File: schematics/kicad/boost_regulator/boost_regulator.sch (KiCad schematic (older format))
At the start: 5 parts, among them SW1 

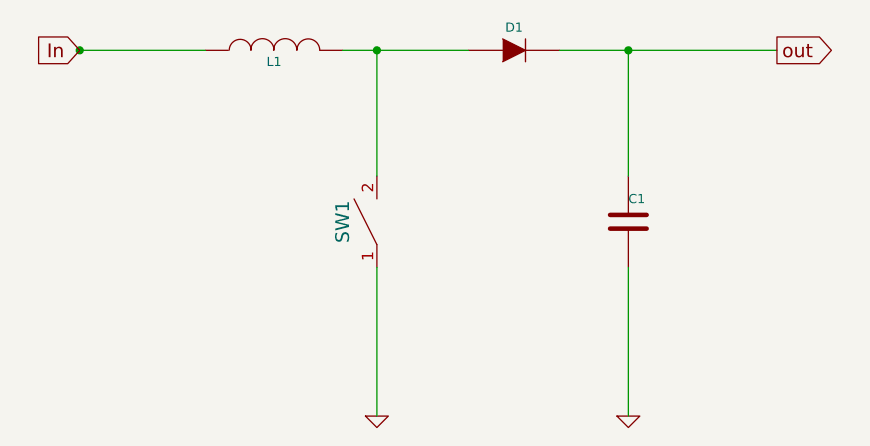
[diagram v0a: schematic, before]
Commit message: schéma jolis pour les screenshot, et screenshots
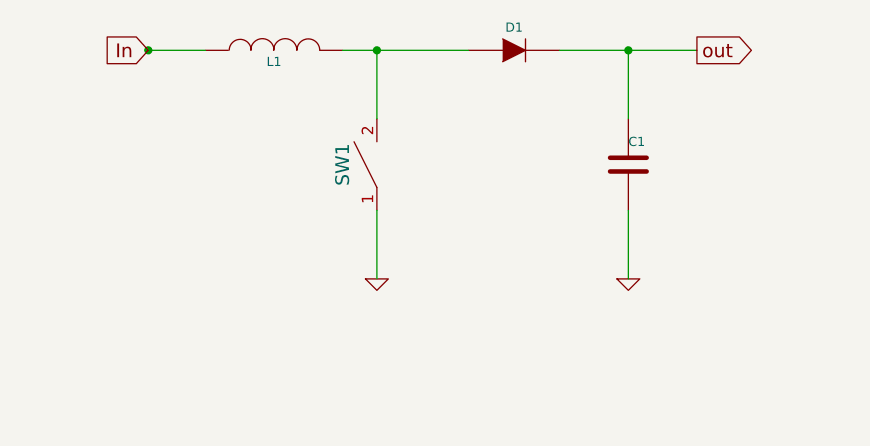
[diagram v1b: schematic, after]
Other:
- moved on the sheet: C1, SW1
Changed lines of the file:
@@
 Sheet 1 1
 Title ""
-Date "8 sep 2015"
+Date "12 sep 2015"
 Rev ""
 Comp ""
@@
 Comment4 ""
 $EndDescr
-Connection ~ 2100 2450
-Text GLabel 2100 2450 0    60   Input ~ 0
+Connection ~ 2400 2450
+Text GLabel 2400 2450 0    60   Input ~ 0
 In
 $Comp
@@
 L C C1
 U 1 1 55EDF250
-P 4500 3200
-F 0 "C1" H 4500 3300 40  0000 L CNN
-F 1 " " H 4506 3115 40  0000 L CNN
-F 2 "~" H 4538 3050 30  0000 C CNN
-F 3 "~" H 4500 3200 60  0000 C CNN
-	1    4500 3200
+P 4500 2950
+F 0 "C1" H 4500 3050 40  0000 L CNN
+F 1 " " H 4506 2865 40  0000 L CNN
+F 2 "~" H 4538 2800 30  0000 C CNN
+F 3 "~" H 4500 2950 60  0000 C CNN
+	1    4500 2950
 	1    0    0    -1
 $EndComp
-Text GLabel 5150 2450 2    60   Output ~ 0
+Text GLabel 4800 2450 2    60   Output ~ 0
 out
 $Comp
 L GND GND
 U 1 1 55EDF277
-P 3400 4050
-F 0 "GND" H 3400 4050 30  0001 C CNN
-F 1 "GND" H 3400 3980 30  0001 C CNN
-F 2 "" H 3400 4050 60  0000 C CNN
-F 3 "" H 3400 4050 60  0000 C CNN
-	1    3400 4050
+P 3400 3450
+F 0 "GND" H 3400 3450 30  0001 C CNN
+F 1 "GND" H 3400 3380 30  0001 C CNN
+F 2 "" H 3400 3450 60  0000 C CNN
+F 3 "" H 3400 3450 60  0000 C CNN
+	1    3400 3450
 	1    0    0    -1
 $EndComp
@@
 L GND #PWR?
 U 1 1 55EDF286
-P 4500 4050
-F 0 "#PWR?" H 4500 4050 30  0001 C CNN
-F 1 "GND" H 4500 3980 30  0001 C CNN
-F 2 "" H 4500 4050 60  0000 C CNN
-F 3 "" H 4500 4050 60  0000 C CNN
-	1    4500 4050
+P 4500 3450
+F 0 "#PWR?" H 4500 3450 30  0001 C CNN
+F 1 "GND" H 4500 3380 30  0001 C CNN
+F 2 "" H 4500 3450 60  0000 C CNN
+F 3 "" H 4500 3450 60  0000 C CNN
+	1    4500 3450
 	1    0    0    -1
 $EndComp
@@
 L SWITCH_SPST SW1
 U 1 1 55EE0317
-P 3400 3200
-F 0 "SW1" H 3400 3350 60  0000 C CNN
-F 1 " " H 3400 3100 60  0000 C CNN
-F 2 "" H 3400 3200 60  0000 C CNN
-F 3 "" H 3400 3200 60  0000 C CNN
-	1    3400 3200
+P 3400 2950
+F 0 "SW1" H 3400 3100 60  0000 C CNN
+F 1 " " H 3400 2850 60  0000 C CNN
+F 2 "" H 3400 2950 60  0000 C CNN
+F 3 "" H 3400 2950 60  0000 C CNN
+	1    3400 2950
 	0    -1   -1   0
 $EndComp
 Wire Wire Line
-	3400 2450 3400 3000
+	3400 2450 3400 2750
 Connection ~ 3400 2450
 Wire Wire Line
-	4200 2450 5150 2450
+	4200 2450 4500 2450
 Wire Wire Line
-	4500 3000 4500 2450
+	4500 2450 4800 2450
+Wire Wire Line
+	4500 2750 4500 2450
 Connection ~ 4500 2450
 Wire Wire Line
-	3400 3400 3400 4050
+	3400 3150 3400 3450
 Wire Wire Line
-	4500 4050 4500 3400
+	4500 3450 4500 3150
 $Comp
 L INDUCTOR L1
@@
 $EndComp
 Wire Wire Line
-	2100 2450 2650 2450
+	2400 2450 2650 2450
 Wire Wire Line
-	3250 2450 3800 2450
+	3250 2450 3400 2450
+Wire Wire Line
+	3400 2450 3800 2450
 $EndSCHEMATC
